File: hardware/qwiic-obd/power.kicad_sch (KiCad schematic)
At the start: 34 parts, among them Q501 DMG2301L, Q502 DMG2301L, Q503 MMBT3906, Q504 DMG2301L, U501 AP63203WU, U502 XC9142B50CMR-G

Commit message: Added initial layout (parts dump)
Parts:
- C508, C509, C512, C513, C514: footprint (none) -> Capacitor_SMD:C_0805_2012Metric_Pad1.18x1.45mm_HandSolder
- L501, L502: footprint (none) -> Inductor_SMD:L_0603_1608Metric_Pad1.05x0.95mm_HandSolder
- U502: footprint SC_50CMR-G_TOR -> UltraLibrarian:XC9142B50CMR-G
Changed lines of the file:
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@@
     (property "Reference" "L502" (id 0) (at 77.47 171.45 90))
     (property "Value" "4.7uH > 1A" (id 1) (at 77.47 173.99 90))
-    (property "Footprint" "" (id 2) (at 77.47 177.8 0)
+    (property "Footprint" "Inductor_SMD:L_0603_1608Metric_Pad1.05x0.95mm_HandSolder" (id 2) (at 77.47 177.8 0)
       (effects (font (size 1.27 1.27)) hide)
     )
@@
     (property "Reference" "L501" (id 0) (at 111.76 102.87 90))
     (property "Value" "3.9uH > 3A" (id 1) (at 111.76 105.41 90))
-    (property "Footprint" "" (id 2) (at 111.76 109.22 0)
+    (property "Footprint" "Inductor_SMD:L_0603_1608Metric_Pad1.05x0.95mm_HandSolder" (id 2) (at 111.76 109.22 0)
       (effects (font (size 1.27 1.27)) hide)
     )
@@
       (effects (font (size 1.27 1.27)) (justify right))
     )
-    (property "Footprint" "" (id 2) (at 115.2652 166.37 0)
+    (property "Footprint" "Capacitor_SMD:C_0805_2012Metric_Pad1.18x1.45mm_HandSolder" (id 2) (at 115.2652 166.37 0)
       (effects (font (size 1.27 1.27)) hide)
     )
@@
       (effects (font (size 1.524 1.524)))
     )
-    (property "Footprint" "SC_50CMR-G_TOR" (id 2) (at 77.47 150.114 0)
+    (property "Footprint" "UltraLibrarian:XC9142B50CMR-G" (id 2) (at 77.47 150.114 0)
       (effects (font (size 1.524 1.524)) hide)
     )
@@
       (effects (font (size 1.27 1.27)) (justify left))
     )
-    (property "Footprint" "" (id 2) (at 60.6552 128.27 0)
+    (property "Footprint" "Capacitor_SMD:C_0805_2012Metric_Pad1.18x1.45mm_HandSolder" (id 2) (at 60.6552 128.27 0)
       (effects (font (size 1.27 1.27)) hide)
     )
@@
       (effects (font (size 1.27 1.27)) (justify left))
     )
-    (property "Footprint" "" (id 2) (at 126.6952 118.11 0)
+    (property "Footprint" "Capacitor_SMD:C_0805_2012Metric_Pad1.18x1.45mm_HandSolder" (id 2) (at 126.6952 118.11 0)
       (effects (font (size 1.27 1.27)) hide)
     )
@@
       (effects (font (size 1.27 1.27)) (justify left))
     )
-    (property "Footprint" "" (id 2) (at 144.4752 118.11 0)
+    (property "Footprint" "Capacitor_SMD:C_0805_2012Metric_Pad1.18x1.45mm_HandSolder" (id 2) (at 144.4752 118.11 0)
       (effects (font (size 1.27 1.27)) hide)
     )
@@
       (effects (font (size 1.27 1.27)) (justify right))
     )
-    (property "Footprint" "" (id 2) (at 46.6852 163.83 0)
-      (effects (font (size 1.27 1.27)) hide)
-    )
+    (property "Footprint" "Capacitor_SMD:C_0805_2012Metric_Pad1.18x1.45mm_HandSolder" (id 2) (at 46.6852 163.83 0)
+      (effects (font (size 1.27 1.27)) hide)
+    )

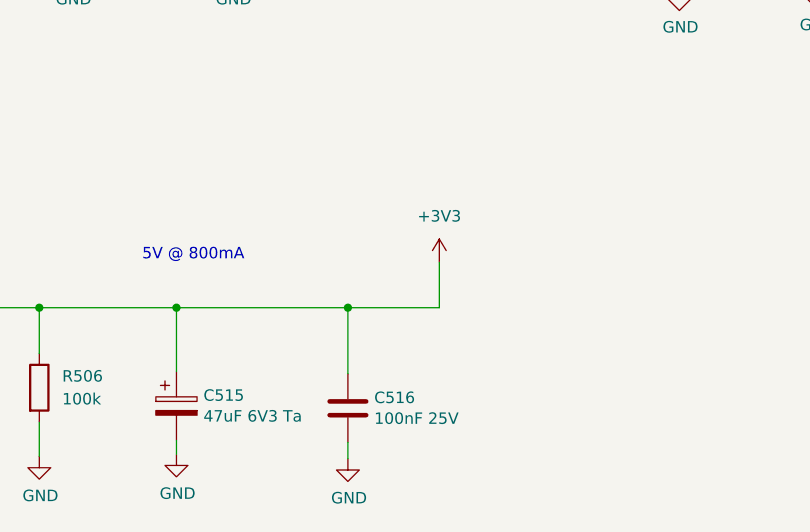
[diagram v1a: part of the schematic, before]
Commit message: OK, layout v1 complete
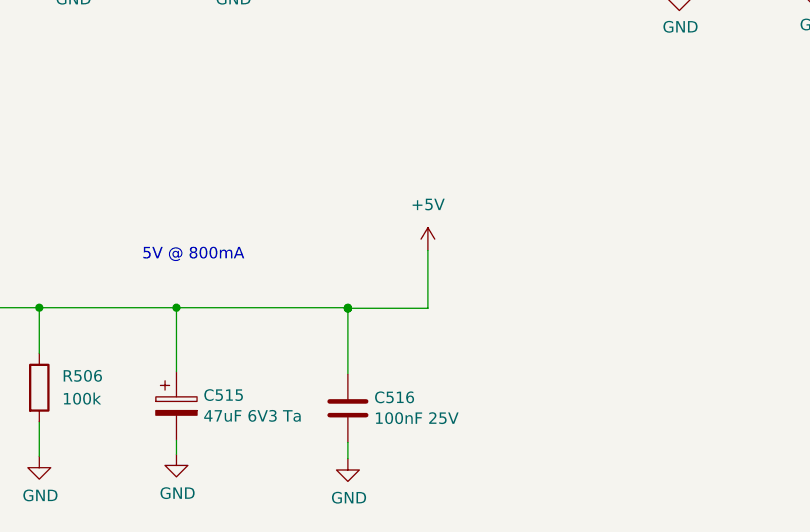
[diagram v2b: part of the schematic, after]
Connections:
- net +3V3: no longer C514.2, C515.1, C516.1, R506.1, U502.4 (VOUT)
- new net +5V: C514.2, C515.1, C516.1, R506.1, U502.4 (VOUT)
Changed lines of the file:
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@@
   (junction (at 97.79 49.53) (diameter 0) (color 0 0 0 0)
   )
+  (junction (at 156.21 161.3913) (diameter 0) (color 0 0 0 0)
+  )
   (junction (at 121.92 161.29) (diameter 0) (color 0 0 0 0)
   )
@@
   (junction (at 231.14 49.53) (diameter 0) (color 0 0 0 0)
   )
+  (junction (at 156.21 161.3555) (diameter 0) (color 0 0 0 0)
+  )
   (junction (at 62.23 61.722) (diameter 0) (color 0 0 0 0)
   )
@@
     (stroke (width 0) (type default) (color 0 0 0 0))
   )
+  (wire (pts (xy 165.1 161.3555) (xy 156.21 161.3555))
+    (stroke (width 0) (type default) (color 0 0 0 0))
+  )
   (wire (pts (xy 241.3 44.45) (xy 241.3 49.53))
     (stroke (width 0) (type default) (color 0 0 0 0))
@@
     (stroke (width 0) (type default) (color 0 0 0 0))
   )
-  (wire (pts (xy 156.21 161.29) (xy 166.37 161.29))
-    (stroke (width 0) (type default) (color 0 0 0 0))
-  )
   (wire (pts (xy 185.42 109.22) (xy 193.04 109.22))
     (stroke (width 0) (type default) (color 0 0 0 0))
@@
     (stroke (width 0) (type default) (color 0 0 0 0))
   )
-  (wire (pts (xy 166.37 156.21) (xy 166.37 161.29))
-    (stroke (width 0) (type default) (color 0 0 0 0))
-  )
   (wire (pts (xy 128.27 59.182) (xy 128.27 60.706))
     (stroke (width 0) (type default) (color 0 0 0 0))
@@
     (stroke (width 0) (type default) (color 0 0 0 0))
   )
+  (wire (pts (xy 165.1 154.94) (xy 165.1 161.3555))
+    (stroke (width 0) (type default) (color 0 0 0 0))
+  )
   (wire (pts (xy 62.23 49.53) (xy 62.23 52.324))
     (stroke (width 0) (type default) (color 0 0 0 0))
@@
     (stroke (width 0) (type default) (color 0 0 0 0))
   )
+  (wire (pts (xy 156.21 161.3555) (xy 156.21 161.3913))
+    (stroke (width 0) (type default) (color 0 0 0 0))
+  )
   (wire (pts (xy 45.72 161.29) (xy 45.72 163.83))
     (stroke (width 0) (type default) (color 0 0 0 0))
@@
     (stroke (width 0) (type default) (color 0 0 0 0))
   )
-  (wire (pts (xy 156.21 161.29) (xy 156.21 168.656))
+  (wire (pts (xy 156.21 161.29) (xy 156.21 161.3555))
     (stroke (width 0) (type default) (color 0 0 0 0))
   )
@@
   )
   (wire (pts (xy 52.07 166.37) (xy 52.07 158.75))
+    (stroke (width 0) (type default) (color 0 0 0 0))
+  )
+  (wire (pts (xy 156.21 161.3913) (xy 156.21 168.656))
     (stroke (width 0) (type default) (color 0 0 0 0))
   )
@@
     (pin "2")
   )
+  (symbol (lib_id "power:+5V") (at 165.1 154.94 0) (unit 1)
+    (in_bom yes) (on_board yes) (fields_autoplaced)
+    (property "Reference" "#PWR0520" (id 0) (at 165.1 158.75 0)
+      (effects (font (size 1.27 1.27)) hide)
+    )
+    (property "Value" "+5V" (id 1) (at 165.1 149.86 0))
+    (property "Footprint" "" (id 2) (at 165.1 154.94 0)
+      (effects (font (size 1.27 1.27)) hide)
+    )
+    (property "Datasheet" "" (id 3) (at 165.1 154.94 0)
+      (effects (font (size 1.27 1.27)) hide)
+    )
+    (pin "1")
+  )
   (symbol (lib_id "Transistor_FET:DMG2301L") (at 184.15 52.07 270) (mirror x) (unit 1)
     (in_bom yes) (on_board yes)
@@
     (pin "2")
   )
-  (symbol (lib_id "power:+3V3") (at 166.37 156.21 0) (unit 1)
-    (in_bom yes) (on_board yes) (fields_autoplaced)
-    (property "Reference" "#PWR0520" (id 0) (at 166.37 160.02 0)
-      (effects (font (size 1.27 1.27)) hide)
-    )
-    (property "Value" "+3V3" (id 1) (at 166.37 151.13 0))
-    (property "Footprint" "" (id 2) (at 166.37 156.21 0)
-      (effects (font (size 1.27 1.27)) hide)
-    )
-    (property "Datasheet" "" (id 3) (at 166.37 156.21 0)
-      (effects (font (size 1.27 1.27)) hide)
-    )
-    (pin "1")
-  )
   (symbol (lib_id "Device:C") (at 143.51 114.3 0) (unit 1)
